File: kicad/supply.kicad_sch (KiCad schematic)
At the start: 26 parts, among them P1 USB_C_Plug_USB2.0, Q3 Si2319CDS, U10 Battery, U11 AP2112K-3.3, U12 LTC4412, U5 TP4056-42-ESOP8, U6 USBLC6-2P6, U7 U8205A, U8 DW01A, U9 Switch

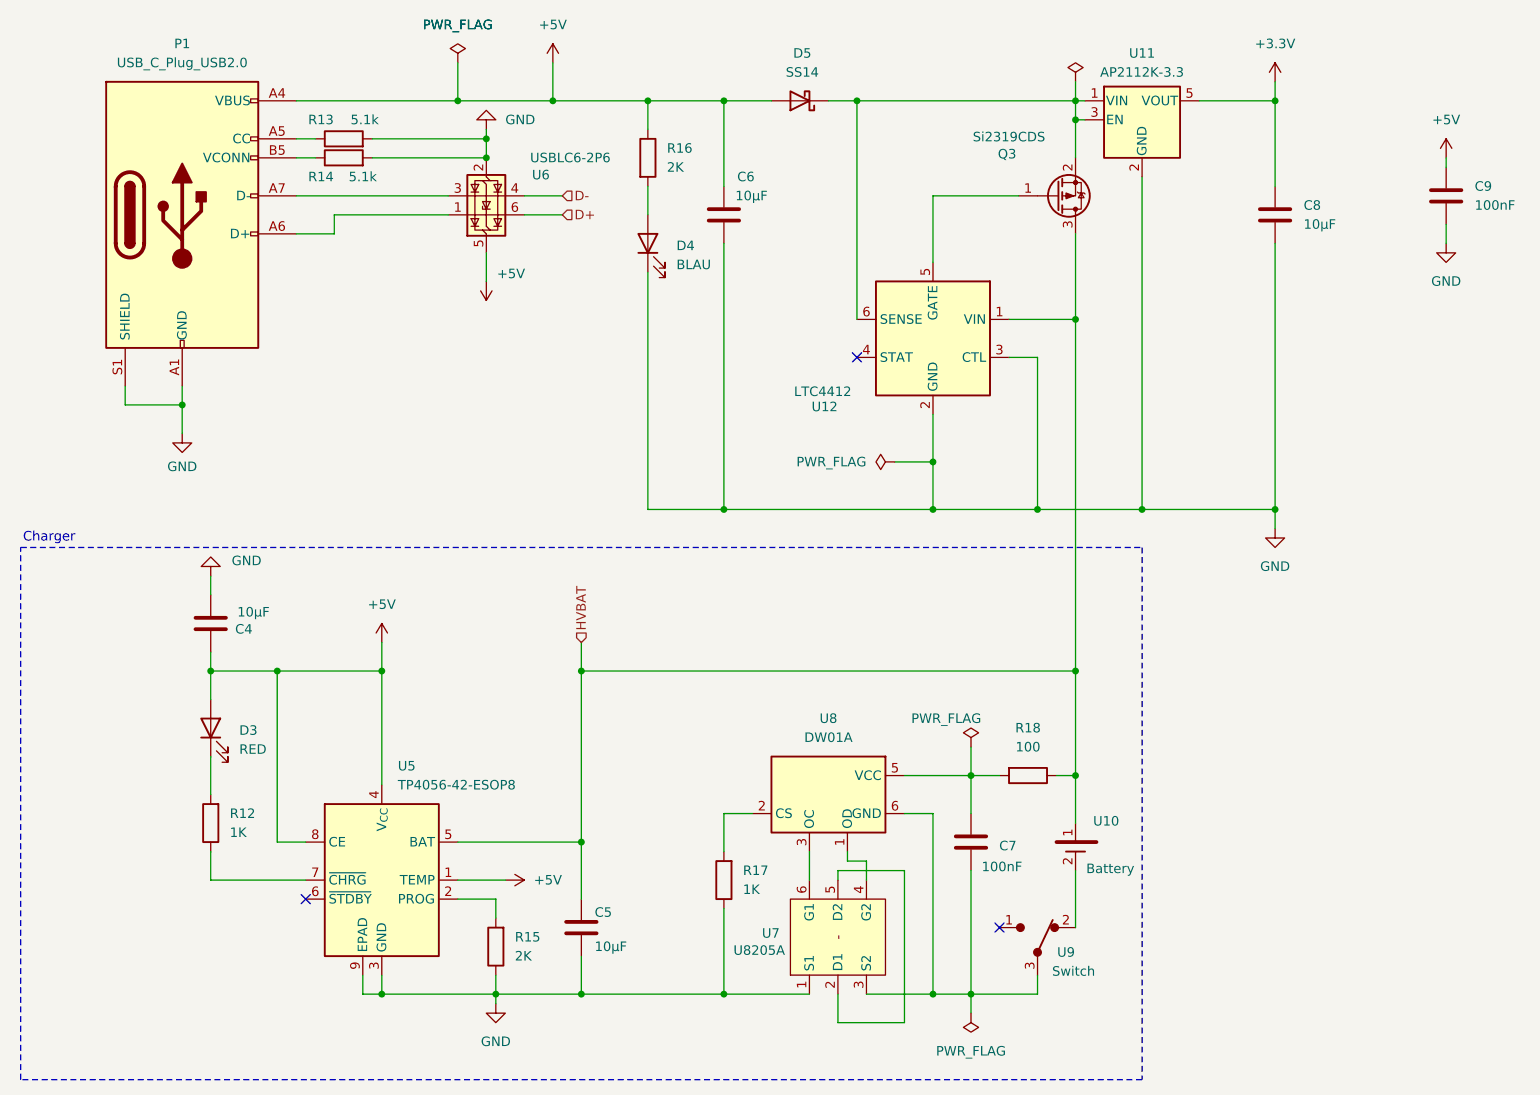
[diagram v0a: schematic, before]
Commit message: docu
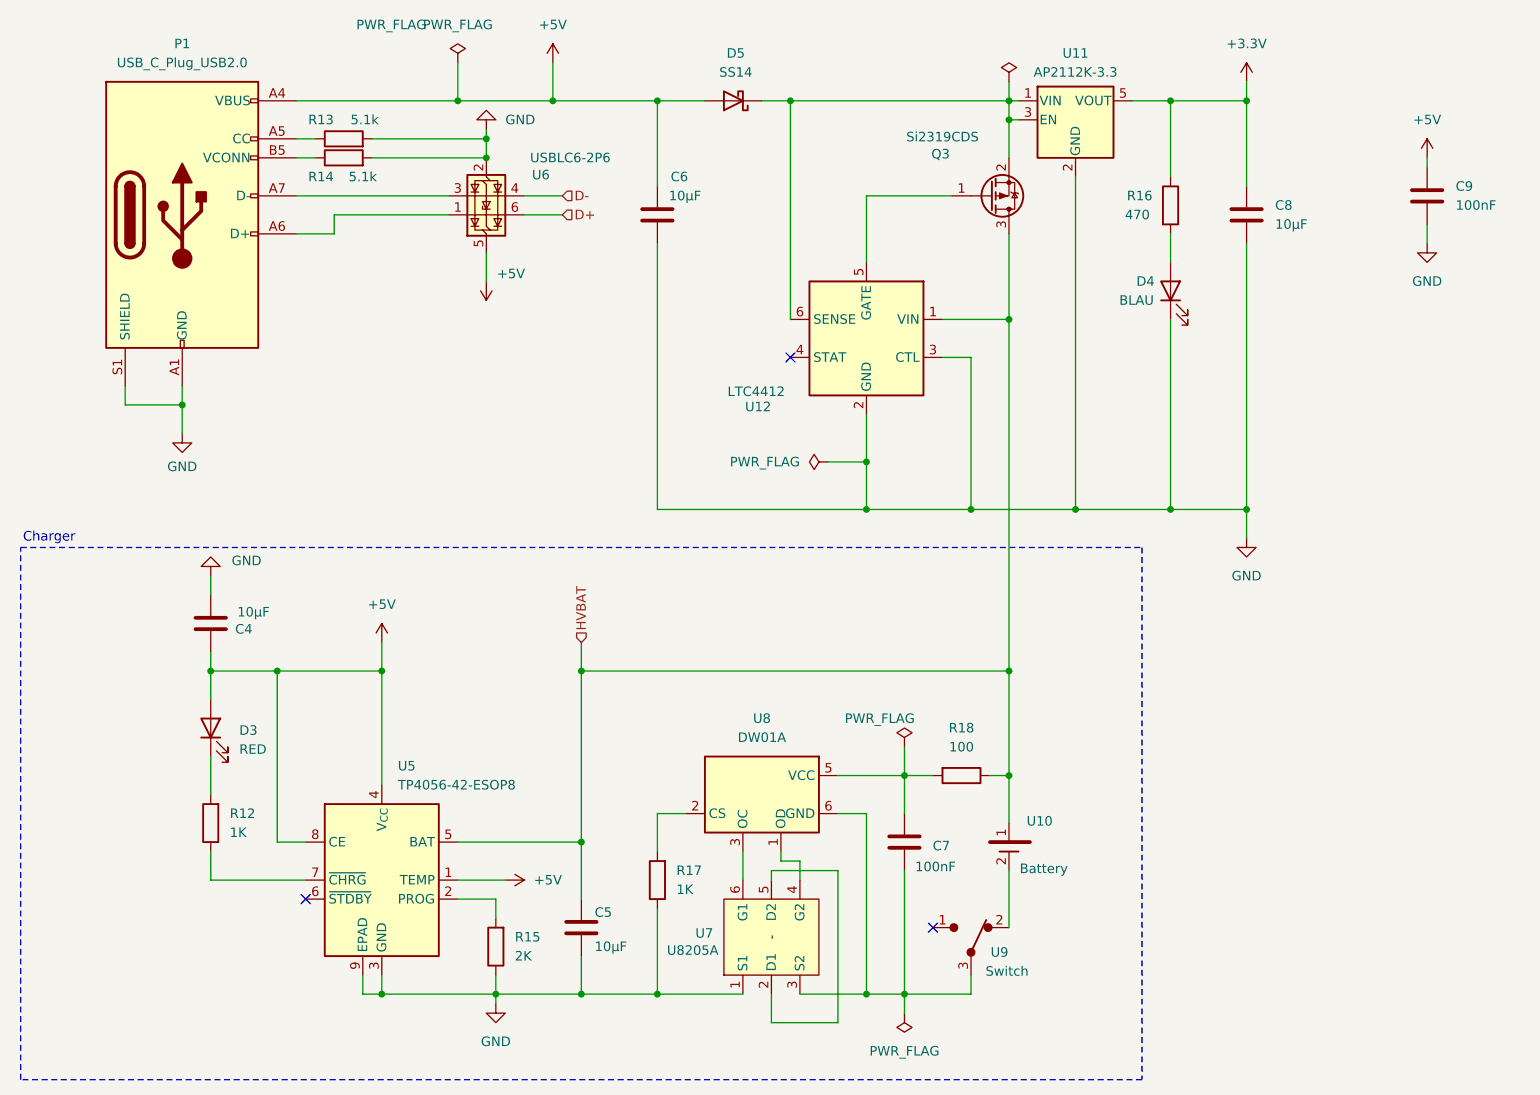
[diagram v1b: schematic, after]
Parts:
- R16: value 2K -> 470
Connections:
- net +3.3V: now also R16.1
- net +5V: no longer R16.1
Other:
- moved on the sheet: C6, C7, C8, C9, D4, D5, Q3, R16, R17, R18, U10, U11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
